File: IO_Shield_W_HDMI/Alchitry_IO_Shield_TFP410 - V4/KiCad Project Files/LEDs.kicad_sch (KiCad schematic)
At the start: 55 parts, among them Q1 Q_PMOS_SGD, Q2 Q_PMOS_SGD, Q3 Q_PMOS_SGD, Q4 Q_PMOS_SGD, SW1 SW_DIP_x08, SW2 SW_DIP_x08, SW3 SW_DIP_x08

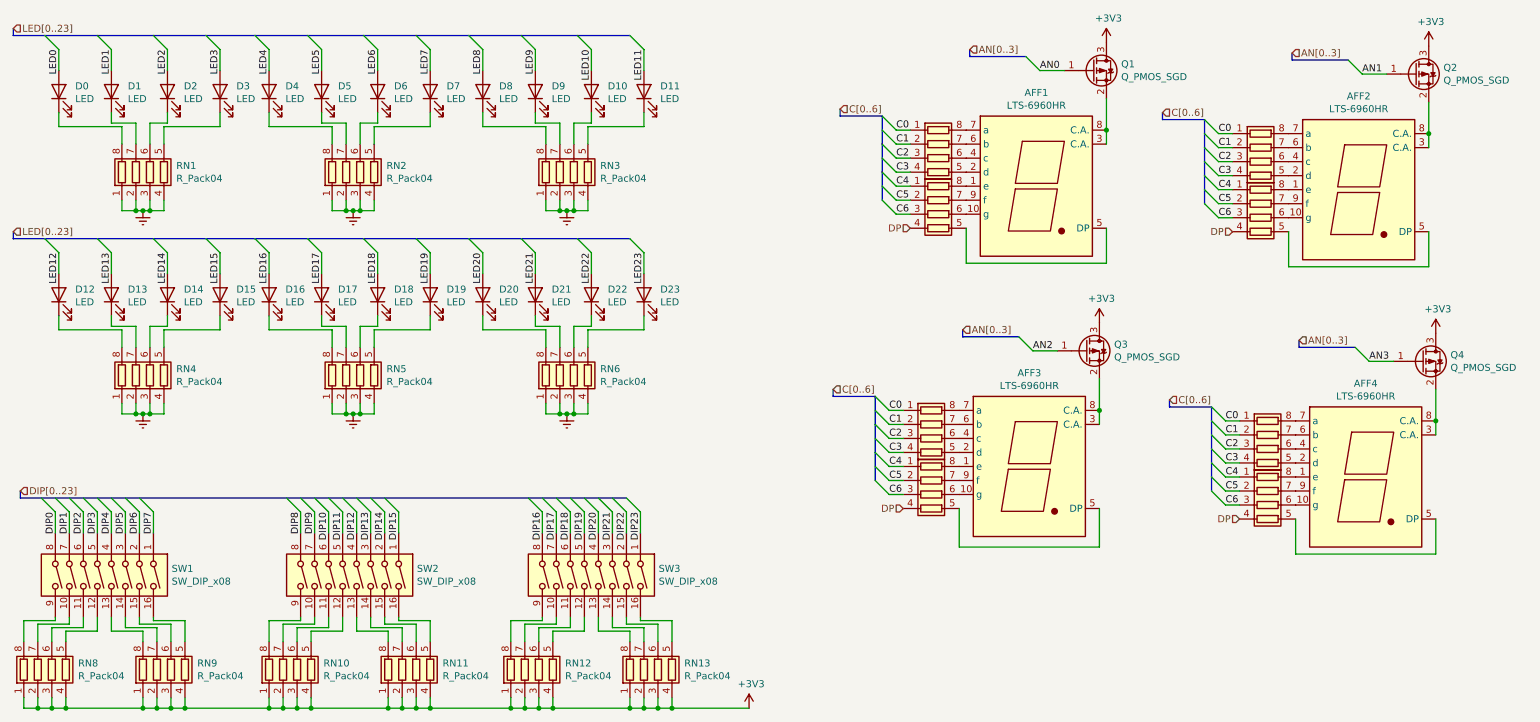
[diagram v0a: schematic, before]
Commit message: minor changes
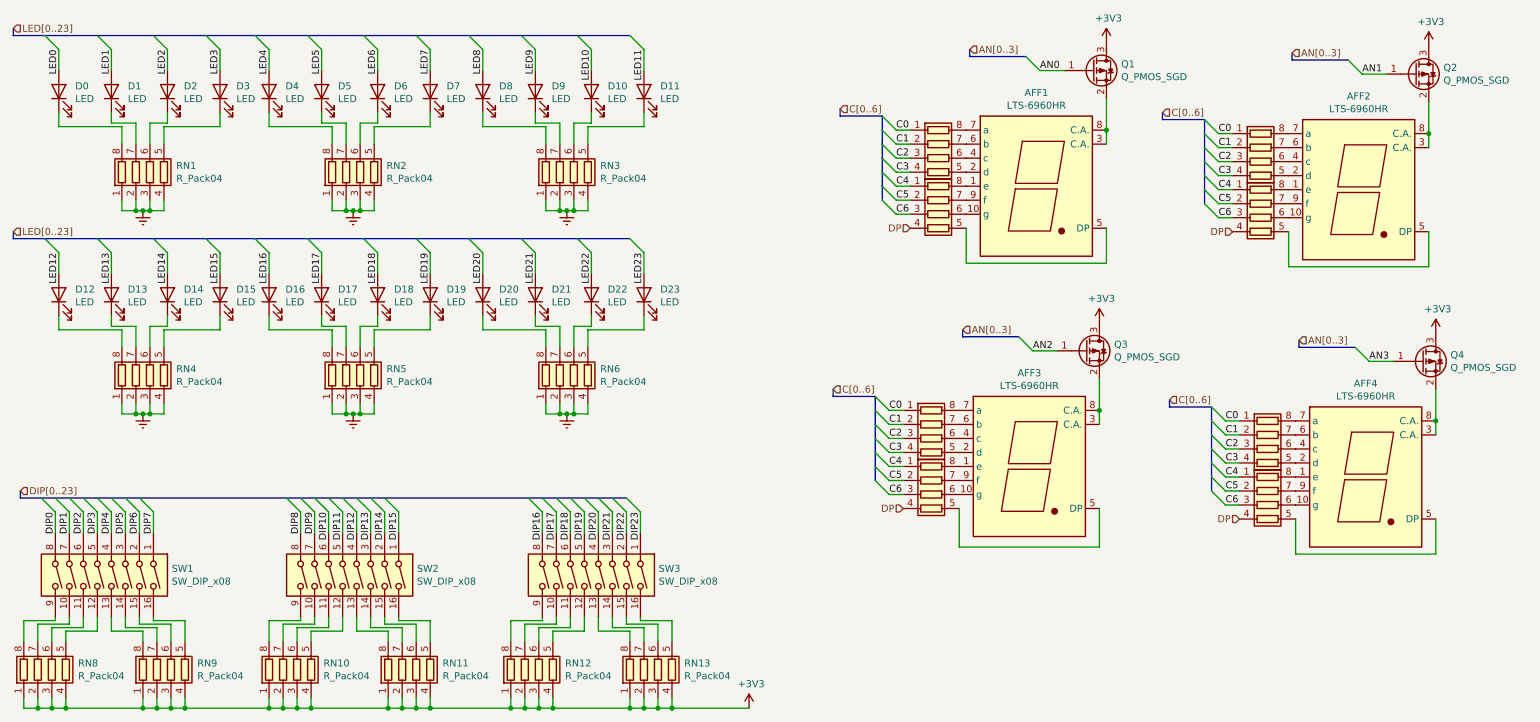
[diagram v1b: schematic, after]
